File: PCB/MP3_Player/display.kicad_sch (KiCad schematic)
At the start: 8 parts, among them Q1 S8050

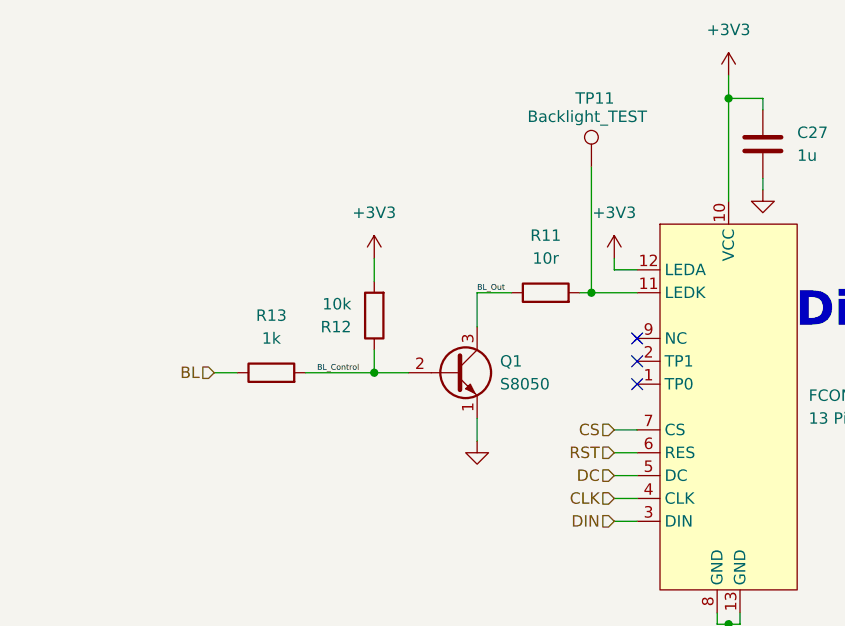
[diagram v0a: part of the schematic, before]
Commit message: Minor Schematic Changes
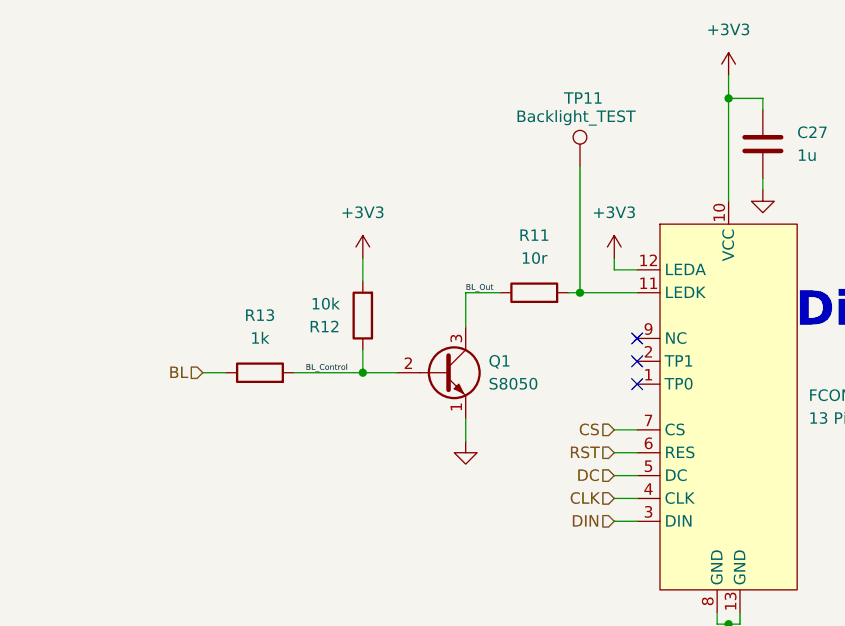
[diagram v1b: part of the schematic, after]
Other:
- moved on the sheet: Q1, R11, R12, R13, TP11
